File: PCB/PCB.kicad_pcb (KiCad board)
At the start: 2 copper layers, 77.6 x 116.7 mm, 39 parts, among them SW1 SW_Push, SW10 SW_Push, SW11 SW_Push, SW12 SW_Push, SW13 SW_Push, SW14 SW_Push, SW15 SW_Push, SW16 SW_Push, SW17 SW_Push, SW2 SW_Push, SW3 SW_Push, SW4 SW_Push, SW5 SW_Push, SW6 SW_Push, SW7 SW_Push, SW8 SW_Push, SW9 SW_Push, U1 XIAO-RP2040-DIP

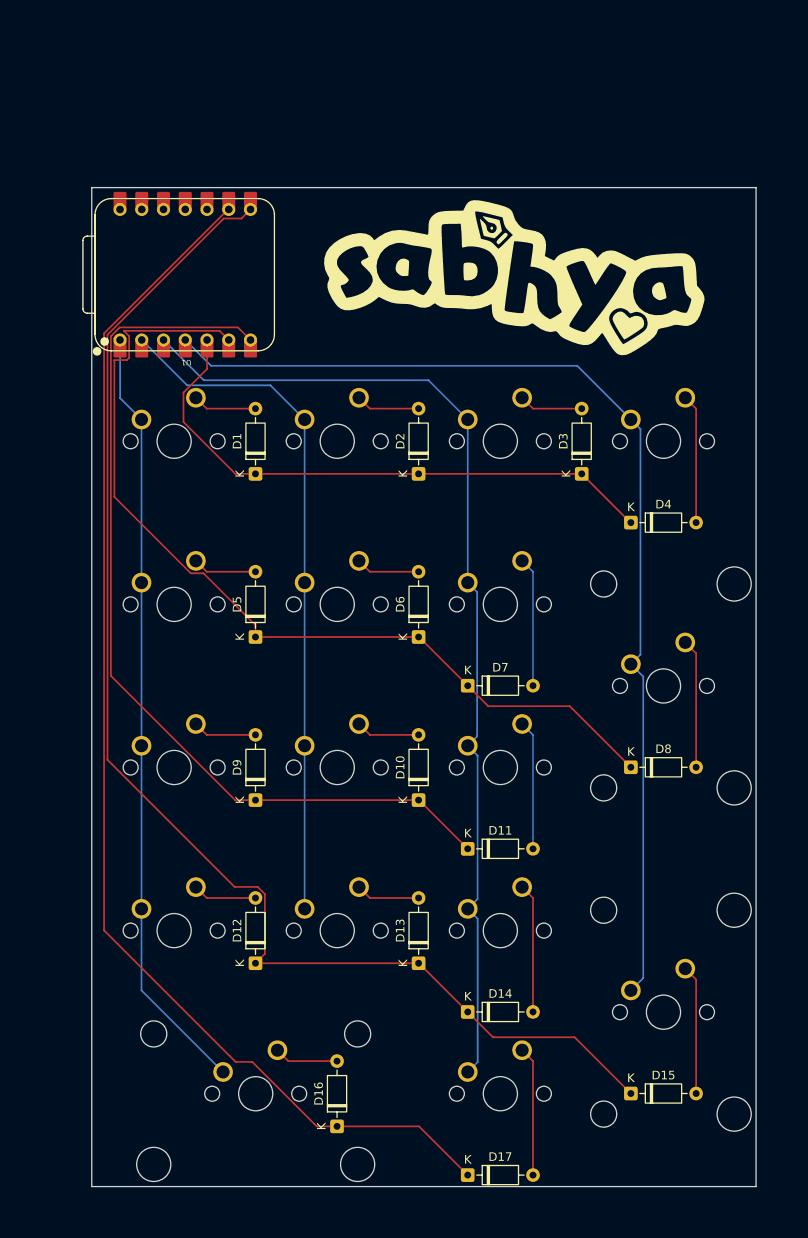
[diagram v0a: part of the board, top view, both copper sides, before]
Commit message: smth
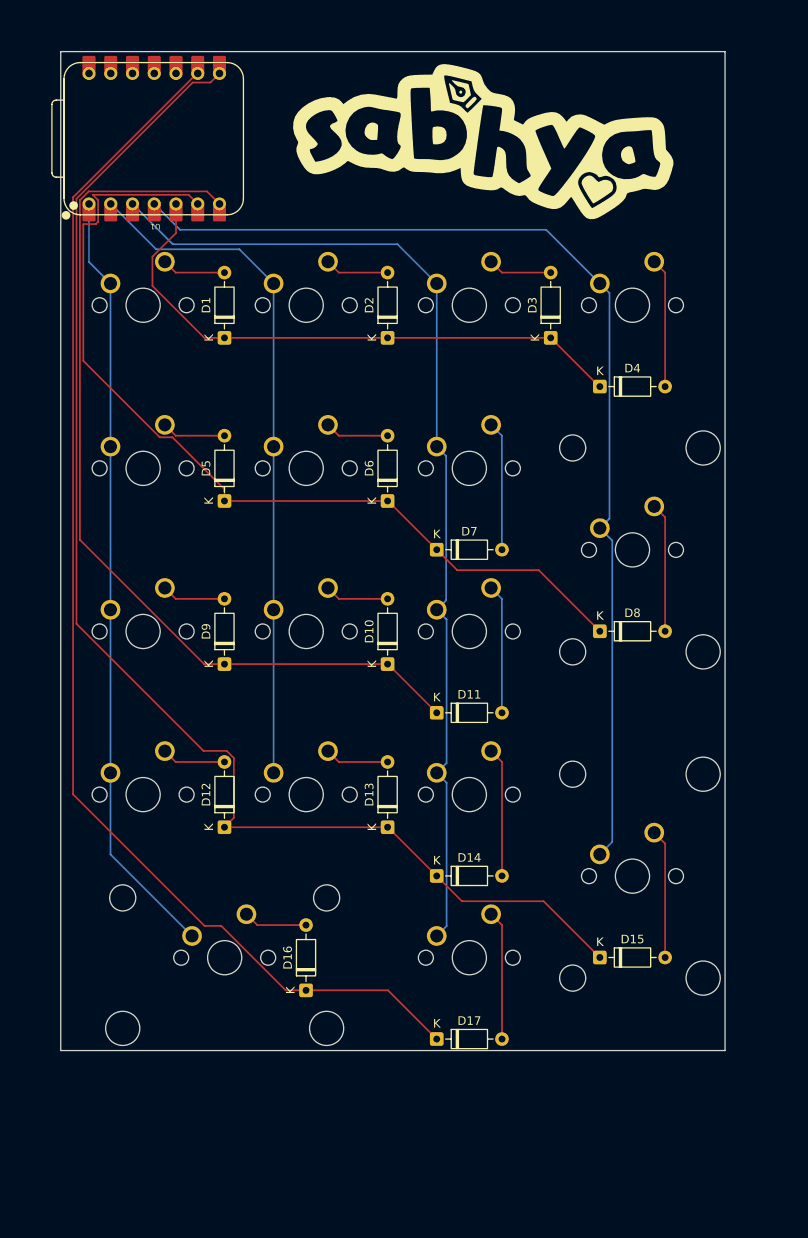
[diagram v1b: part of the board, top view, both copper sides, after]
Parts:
- moved D11 16.3 mm to (141.8, 118.4)
- moved D3 16.3 mm to (155.1, 74.6)
- moved D8 16.3 mm to (160.8, 108.9)
- moved S8 16.3 mm to (164.6, 99.4)
- moved SW11 16.3 mm to (145.6, 108.9)
- moved SW8 16.3 mm to (164.6, 99.4)
- moved D1 16.3 mm to (117.0, 74.6)
- moved D9 16.3 mm to (117.0, 112.7)
- moved SW9 16.3 mm to (107.5, 108.9)
- moved D10 16.3 mm to (136.0, 112.7)
- moved D2 16.3 mm to (136.0, 74.6)
- moved SW10 16.3 mm to (126.5, 108.9)
- moved D14 16.3 mm to (141.8, 137.4)
- moved D15 16.3 mm to (160.8, 147.0)
- moved D16 16.3 mm to (126.5, 150.8)
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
